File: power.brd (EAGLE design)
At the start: 71.8 x 54.6 mm, 22 parts

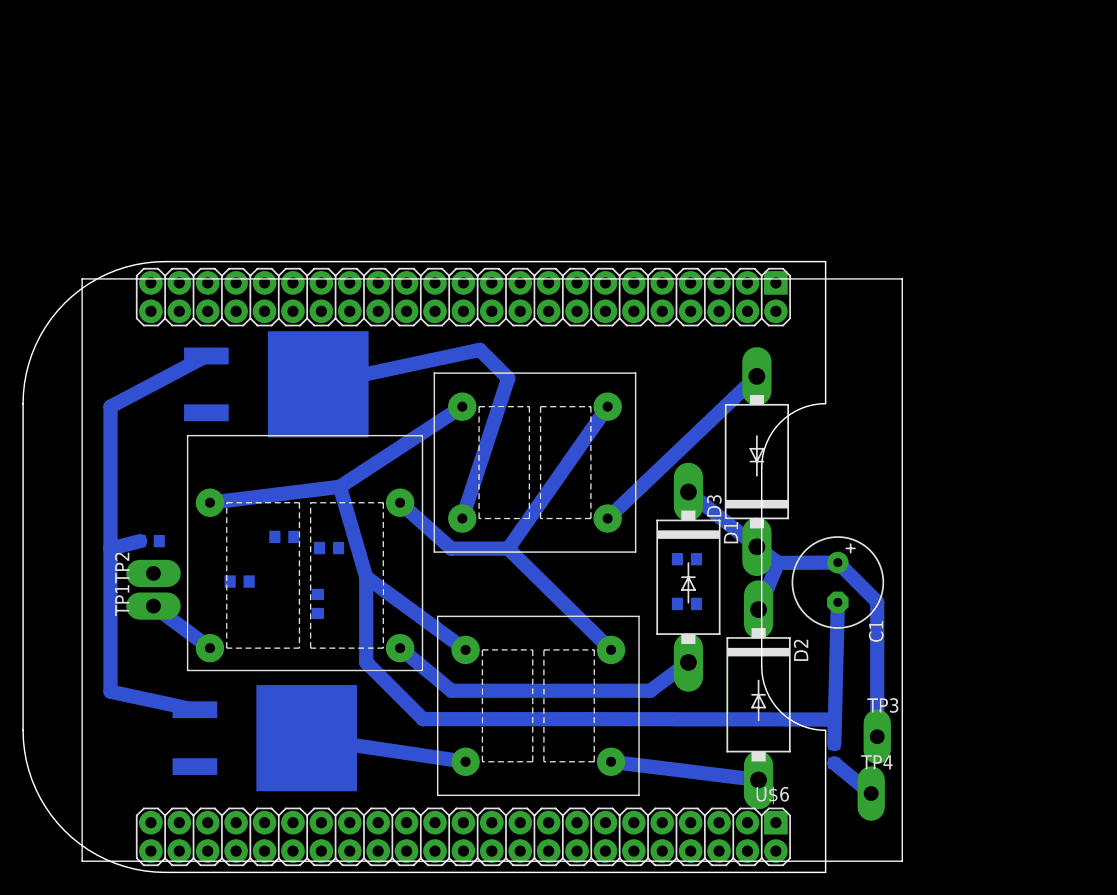
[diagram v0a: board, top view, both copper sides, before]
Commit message: change all the things
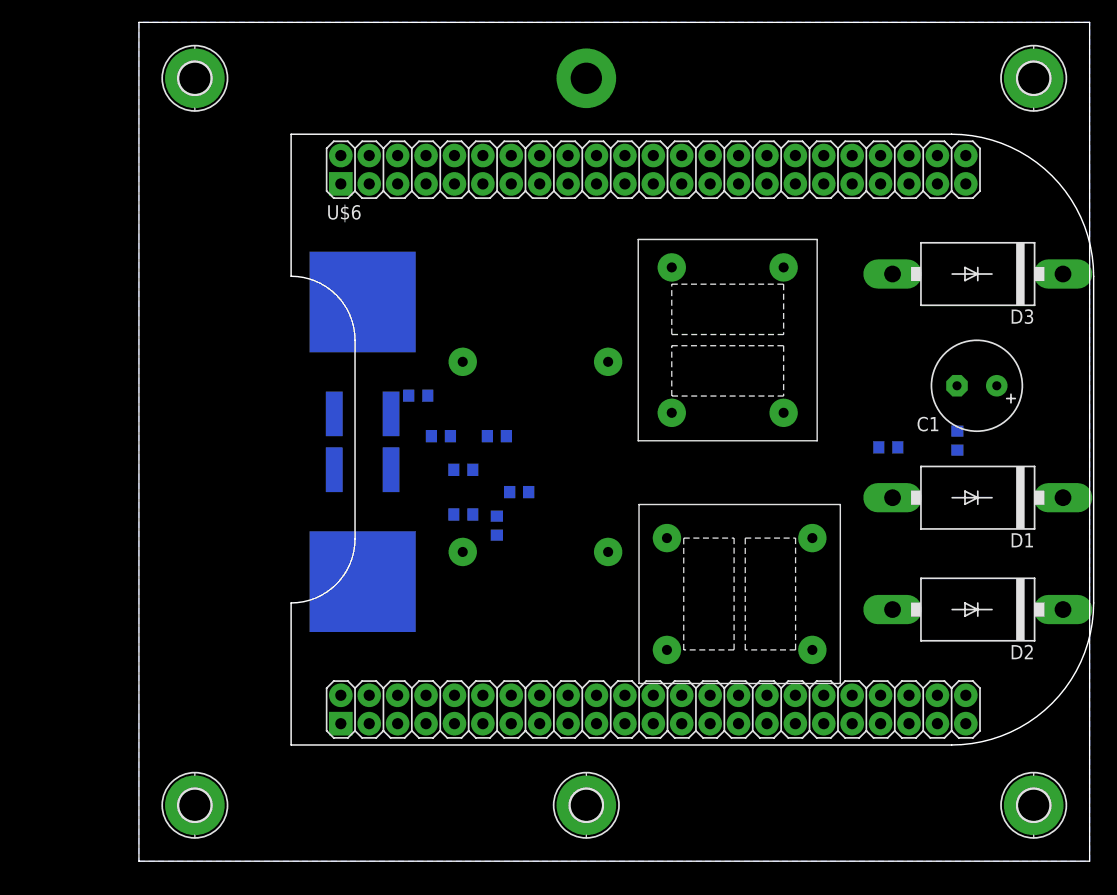
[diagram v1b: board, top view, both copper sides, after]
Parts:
- removed TP1, TP2, TP3, TP4: TPPAD1-13Y, testpad:P1-13Y
- added BAT+, BAT-, H1, H2, PV+, PV-: MOUNT-PAD-ROUND2.8, holes:2,8-PAD
- added R10: 1k, rcl:R0603
- added R9: 47k, rcl:R0603
- R1, R2: value (none) -> 0R1
- moved U$6 101.4 mm to (-1.00, 65.0), turned to 270 degrees
- moved U$3 43.8 mm to (42.0, 44.6), flipped to the bottom, turned to 270 degrees
- moved R1 30.1 mm to (73.2, 37.6)
- moved R2 27.3 mm to (25.0, 41.6)
- moved D1 26.8 mm to (75.0, 32.5), turned to 180 degrees
- moved D3 25.9 mm to (75.0, 52.5), turned to 180 degrees
- moved C1 21.5 mm to (74.9, 42.5), turned to 180 degrees
- moved D2 21.0 mm to (75.0, 22.5), turned to 180 degrees
- moved R3 20.9 mm to (29.0, 31.0), turned to 180 degrees
- moved R7 20.6 mm to (67.0, 37.0)
- moved R8 20.6 mm to (67.0, 33.0)
- moved U$5 20.6 mm to (47.2, 18.9)
- moved R6 18.0 mm to (32.0, 38.0)
- moved R4 17.5 mm to (32.0, 30.0)
- moved R5 16.6 mm to (27.0, 38.0)
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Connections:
- new net N$18: R10.2, R9.2, U$6.79
- new net N$8: R9.1
- net GND: now also H1.B2,8, H2.B2,8, R10.1
- net N$14: now also BAT-.B2,8; no longer TP4.TP
- net N$16: now also PV-.B2,8; no longer TP2.TP
- net N$3: now also PV+.B2,8, U$3.P$3; no longer TP1.TP, U$3.P$1
- net N$6: now also U$3.P$1; no longer U$3.P$3
- net N$7: now also BAT+.B2,8; no longer TP3.TP
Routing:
- net GND: track 108.5 -> 0.00 mm
- net N$11: track 45.6 -> 0.00 mm
- net N$6: track 39.6 -> 0.00 mm
- net N$7: track 37.1 -> 0.00 mm
- net N$5: track 31.6 -> 0.00 mm
- net N$1: track 28.0 -> 0.00 mm
- net N$9: track 18.4 -> 0.00 mm
- net N$15: track 14.4 -> 0.00 mm
- net N$2: track 13.3 -> 0.00 mm
- net N$3: track 6.30 -> 0.00 mm
- net N$14: track 4.27 -> 0.00 mm
- added copper zone on layer 16, net GND
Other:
- board size 71.8 x 54.6 mm -> 85 x 75 mm
